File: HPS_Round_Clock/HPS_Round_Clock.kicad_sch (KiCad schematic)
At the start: 4 parts

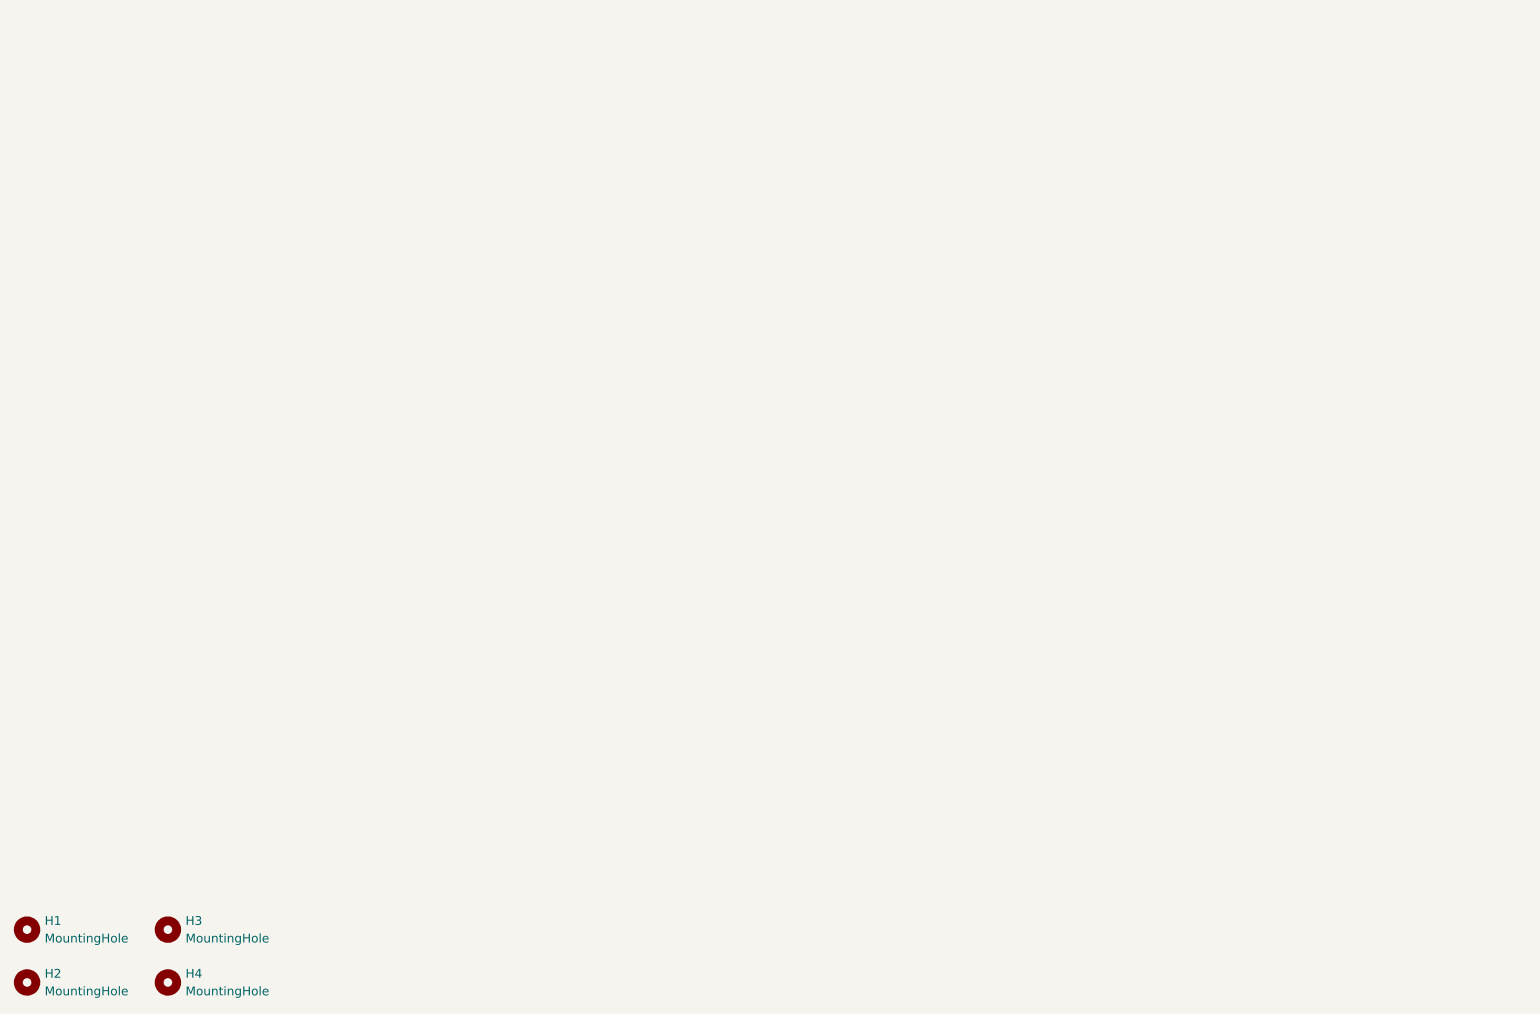
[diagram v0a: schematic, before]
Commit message: Update HPS_Round_Clock.kicad_sch
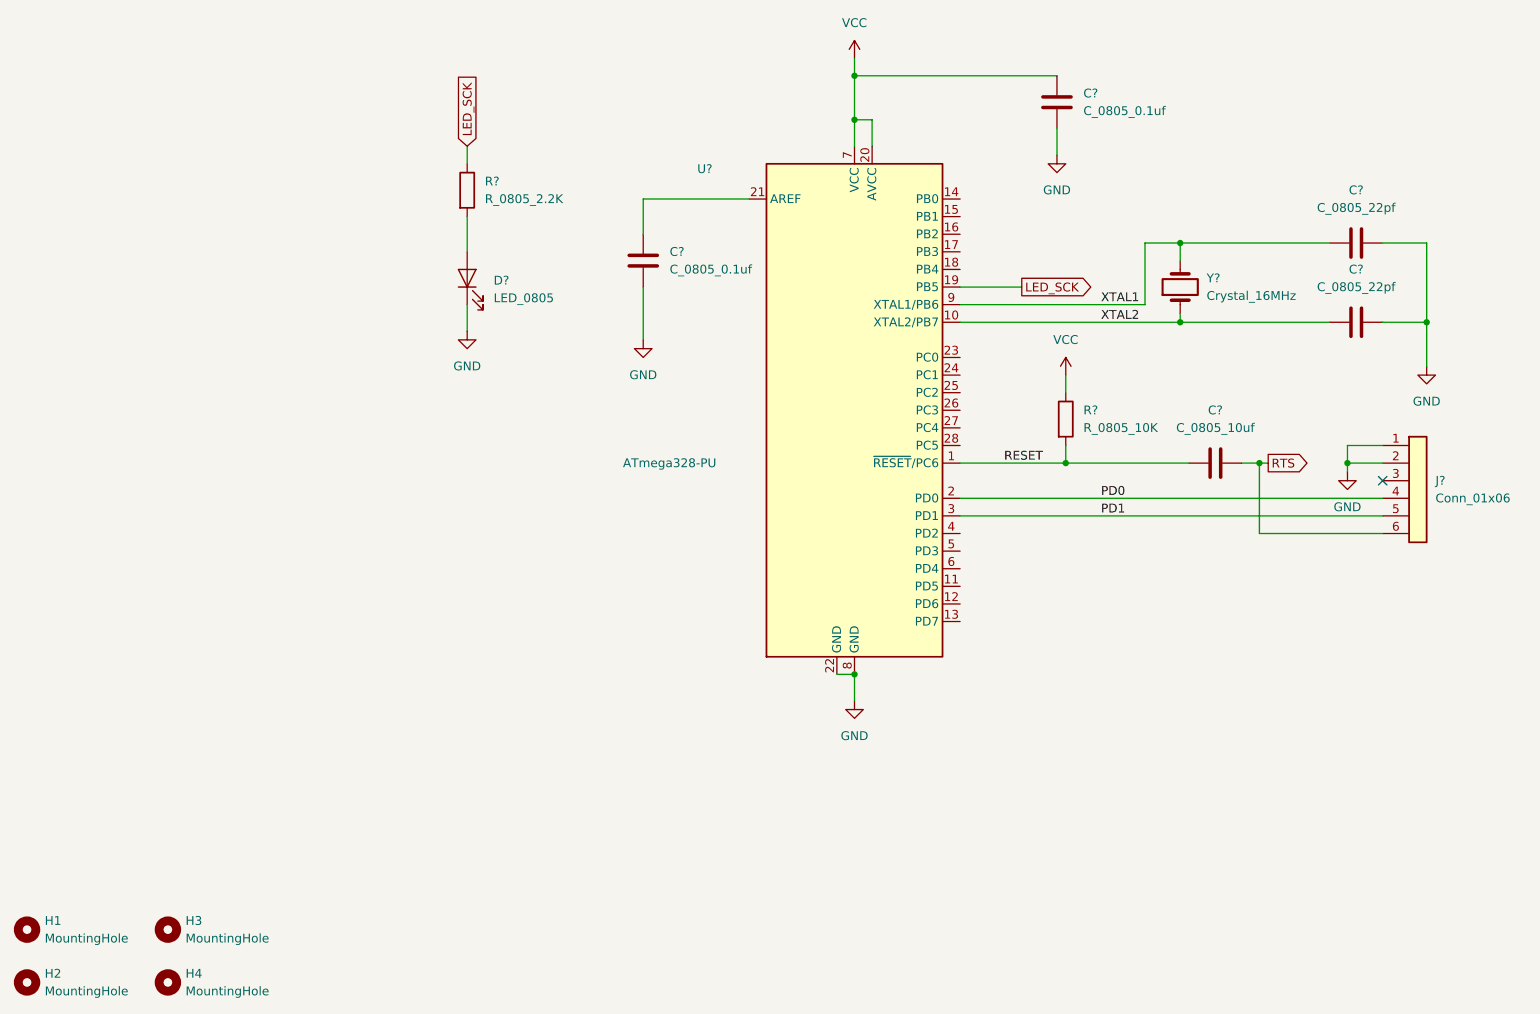
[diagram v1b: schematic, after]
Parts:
- added C? (x2): C_0805_22pf, footprints:C_0805_2012Metric, symbol HPS:C_0805_22pf
- added C? (x2): C_0805_0.1uf, footprints:C_0805_2012Metric, symbol HPS:C_0805_0.1uf
- added C?: C_0805_10uf, footprints:C_0805_2012Metric, symbol HPS:C_0805_10uf
- added D?: LED_0805, footprints:LED_0805_2012Metric, symbol HPS:LED_0805
- added J?: Conn_01x06, footprints:PinHeader_1x06_P2.54mm_Vertical, symbol HPS:Conn_01x06
- added R?: R_0805_10K, footprints:R_0805_2012Metric, symbol HPS:R_0805_10K
- added R?: R_0805_2.2K, footprints:R_0805_2012Metric, symbol HPS:R_0805_2.2K
- added U?: ATmega328-PU, footprints:DIP-28_W7.62mm, symbol HPS:ATmega328-PU
- added Y?: Crystal_16MHz, footprints:Crystal_SMD_HC49-SD, symbol HPS:Crystal_16MHz
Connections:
- new net: D?.2 (A), R?.2
- new net: C?.1, U?.21 (AREF)
- new net GND: C?.1, C?.1, C?.2, C?.2, D?.1 (K), J?.1 (Pin_1), J?.2 (Pin_2), U?.22 (GND), U?.8 (GND)
- new net LED_SCK: R?.1, U?.19 (PB5)
- new net PD0: J?.4 (Pin_4), U?.2 (PD0)
- new net PD1: J?.5 (Pin_5), U?.3 (PD1)
- new net RESET: C?.1, R?.2, U?.1 (~{RESET}/PC6)
- new net RTS: C?.2, J?.6 (Pin_6)
- new net VCC: C?.1, R?.1, U?.20 (AVCC), U?.7 (VCC)
- new net XTAL1: C?.2, U?.9 (XTAL1/PB6), Y?.2
- new net XTAL2: C?.2, U?.10 (XTAL2/PB7), Y?.1
- no-connect marks 0 -> 1
